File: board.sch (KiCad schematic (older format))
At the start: 0 parts

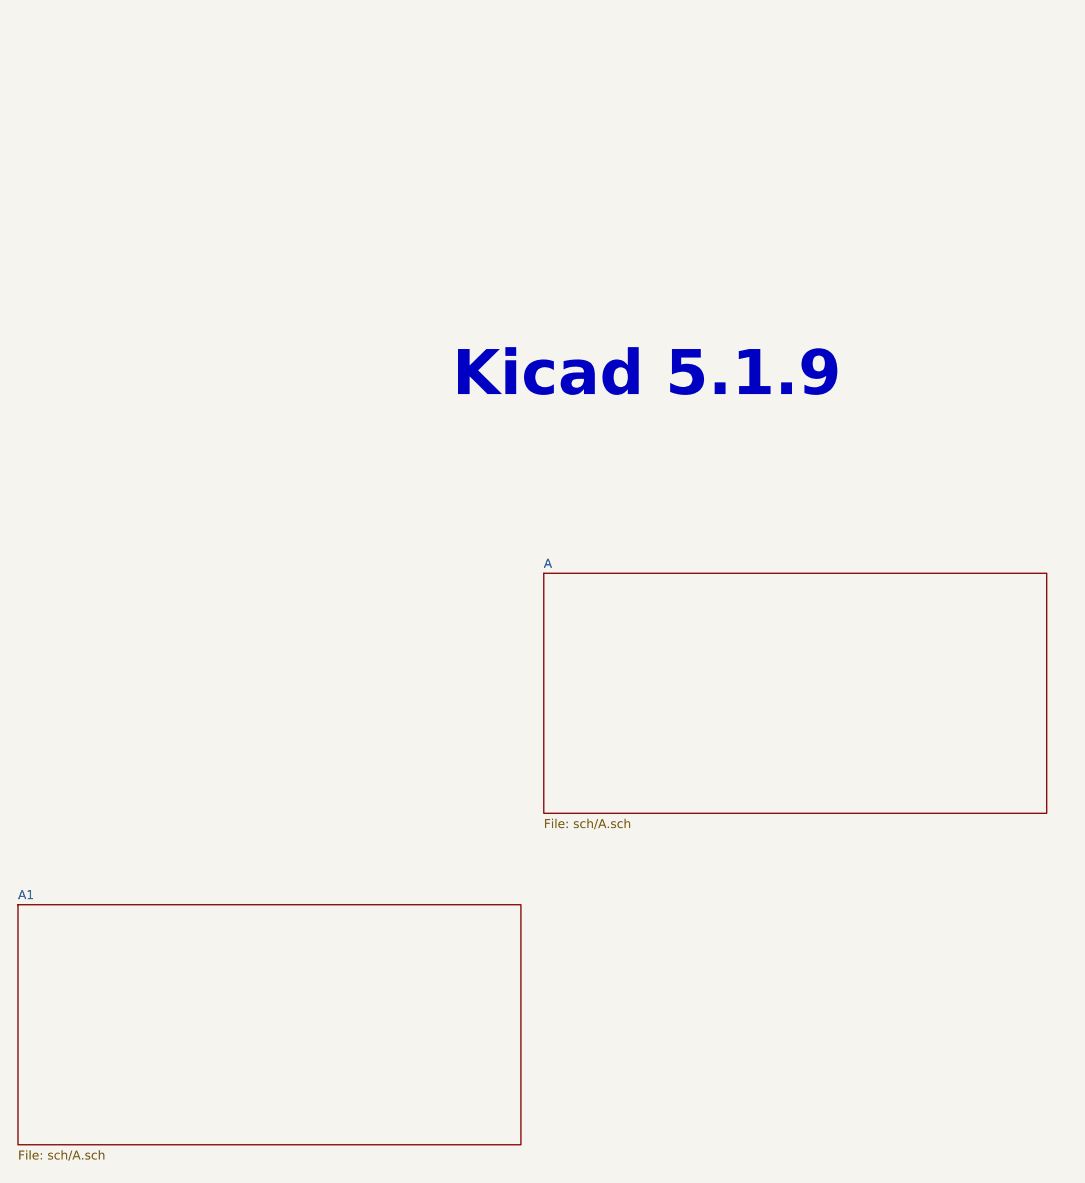
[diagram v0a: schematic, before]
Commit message: Update
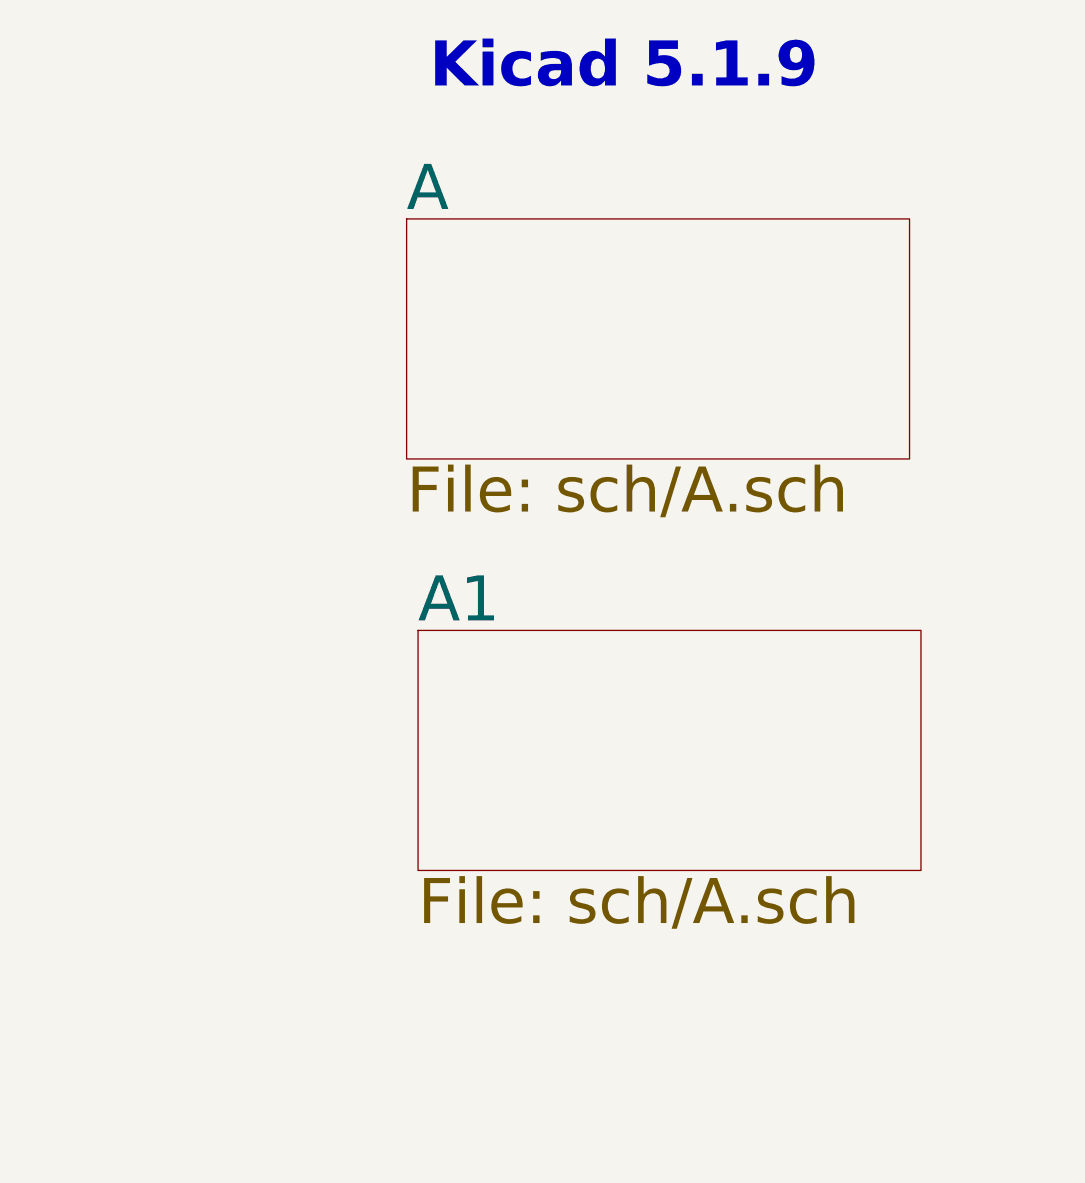
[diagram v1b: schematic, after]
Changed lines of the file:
@@
 $Descr A4 11693 8268
 encoding utf-8
-Sheet 1 5
+Sheet 1 9
 Title ""
 Date ""
@@
 Comment4 ""
 $EndDescr
-Text Notes 5200 3150 0    197  ~ 39
+Text Notes 5100 1800 0    197  ~ 39
 Kicad 5.1.9
 $Sheet
-S 5600 3900 2200 1050
+S 5000 2350 2200 1050
 U 62CDCBF7
-F0 "A" 39
-F1 "sch/A.sch" 39
+F0 "A" 197
+F1 "sch/A.sch" 197
 $EndSheet
 $Sheet
-S 3300 5350 2200 1050
+S 5050 4150 2200 1050
 U 62CDD692
-F0 "A1" 39
-F1 "sch/A.sch" 39
+F0 "A1" 197
+F1 "sch/A.sch" 197
 $EndSheet
 $EndSCHEMATC
